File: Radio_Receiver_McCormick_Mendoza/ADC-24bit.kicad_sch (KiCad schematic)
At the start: 14 parts, among them U12 PCM1808PWR

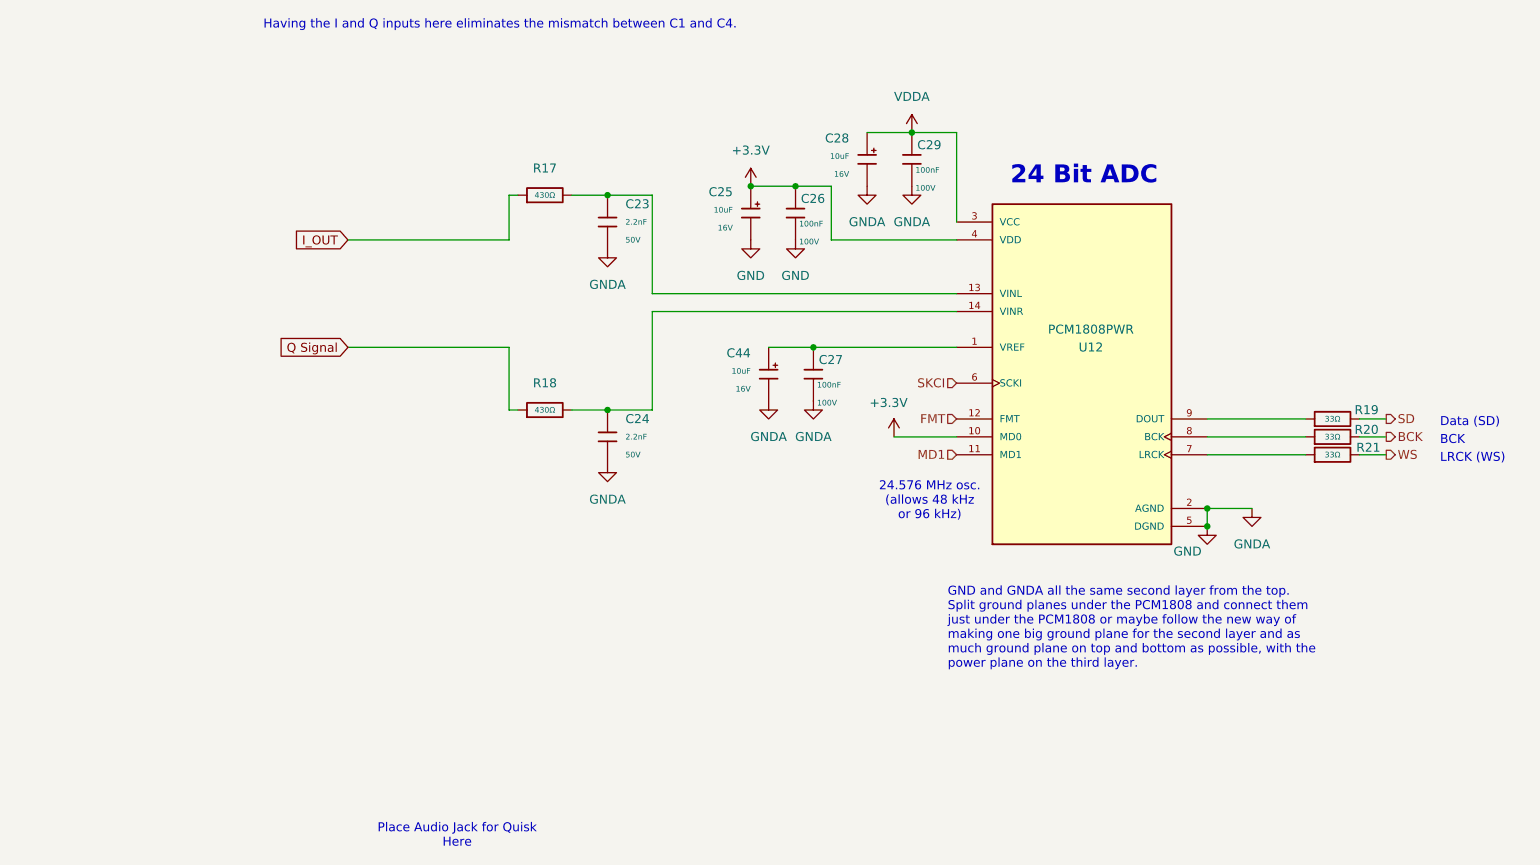
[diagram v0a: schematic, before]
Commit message: Schematic edits power and signal systems
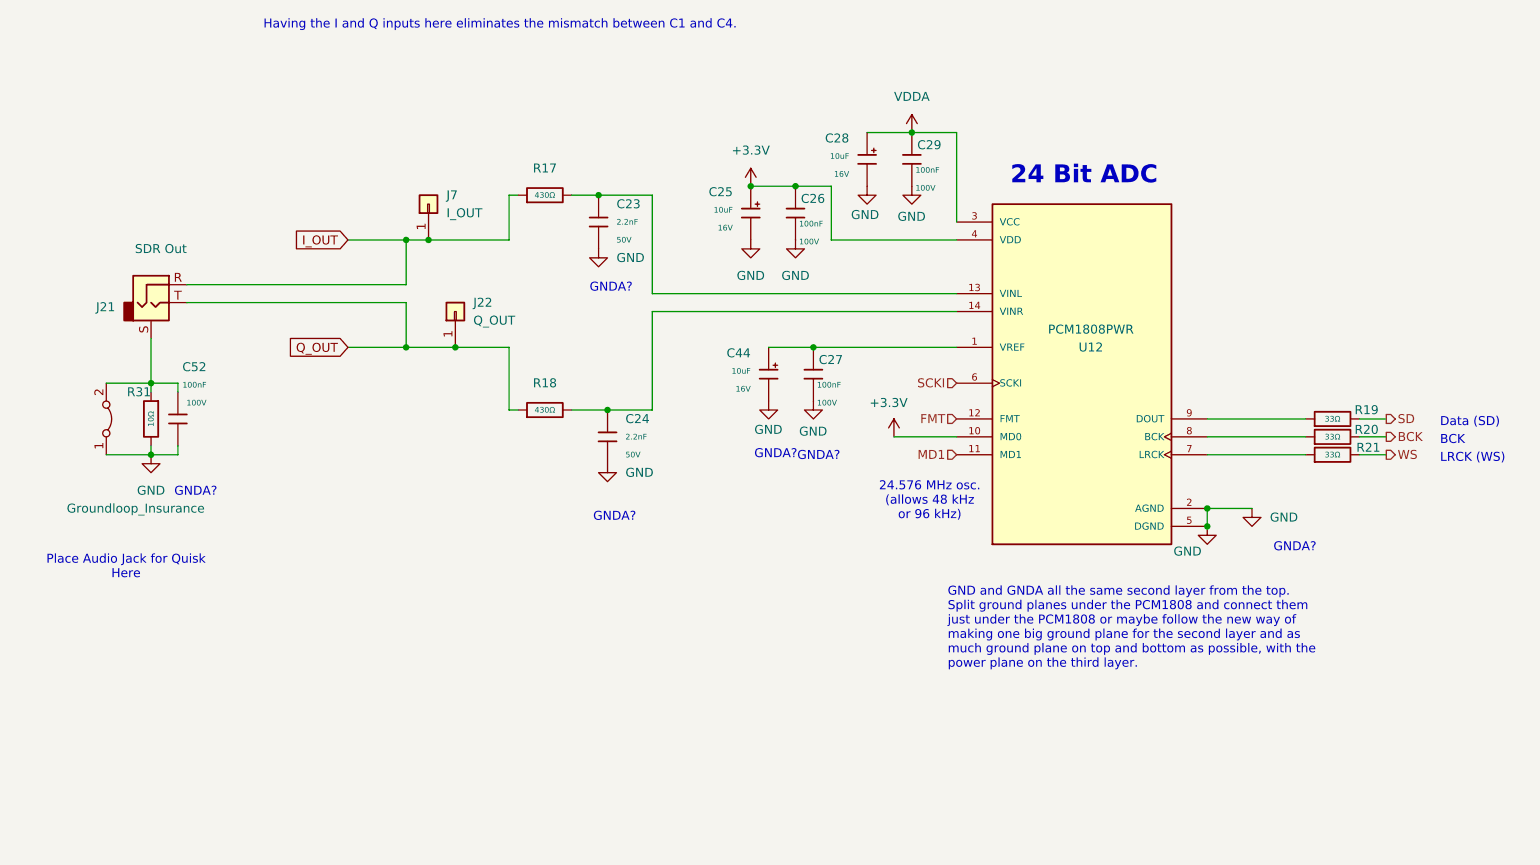
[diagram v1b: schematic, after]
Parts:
- added C52: 100nF, PCM_JLCPCB:C_0805, symbol PCM_JLCPCB-Capacitors:0805,100nF
- added J21: SDR Out, Intro_to_CAD:Jack_3.5mm_CUI_SJ-3523-SMT_Horizontal, symbol Connector_Audio:AudioJack2_Ground
- added J22: Q_OUT, Connector_PinHeader_2.54mm:PinHeader_1x01_P2.54mm_Vertical, symbol Connector_Generic:Conn_01x01
- added J7: I_OUT, Connector_PinHeader_2.54mm:PinHeader_1x01_P2.54mm_Vertical, symbol Connector_Generic:Conn_01x01
- added R31: 10Ω, PCM_JLCPCB:R_0603, symbol PCM_JLCPCB-Resistors:0603,10Ω
- added e5: Groundloop_Insurance, Jumper:SolderJumper-2_P1.3mm_Bridged_RoundedPad1.0x1.5mm, symbol Jumper:Jumper_2_Bridged
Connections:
- net GND: now also C52.1, R31.2, e5.1 (A)
- net I_OUT: now also J21.R, J7.1 (Pin_1)
- net Q Signal renamed Q_OUT
- net Q_OUT: now also J21.T, J22.1 (Pin_1)
- net SKCI renamed SCKI
- new net: C52.2, J21.S, R31.1, e5.2 (B)
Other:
- note added: "GNDA?"
- moved on the sheet: C23
